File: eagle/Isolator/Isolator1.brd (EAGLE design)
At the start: 100 x 80 mm, 15 parts, among them J1 61300411121, J2 61300411121, J4 PJ-102A, Q1 BC557C, Q2 BC557C

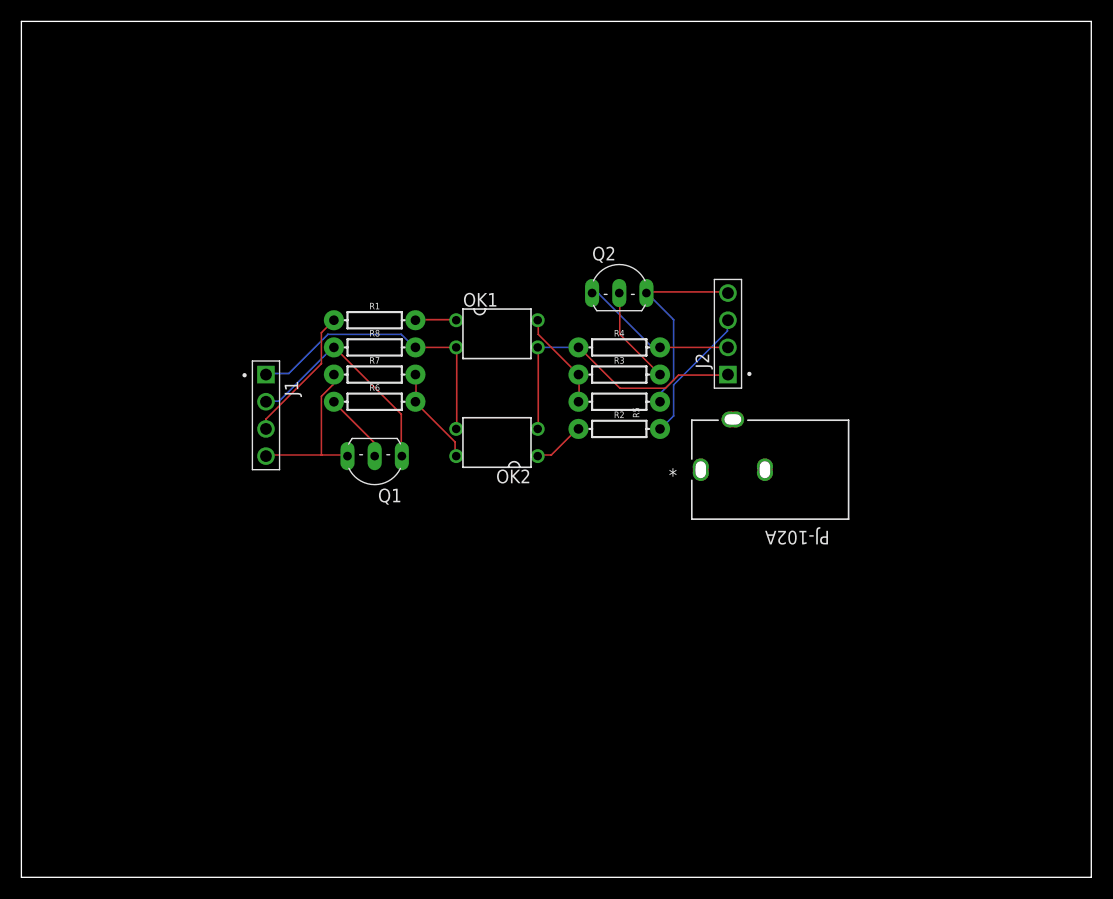
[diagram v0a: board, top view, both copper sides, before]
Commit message: Working - check power jack
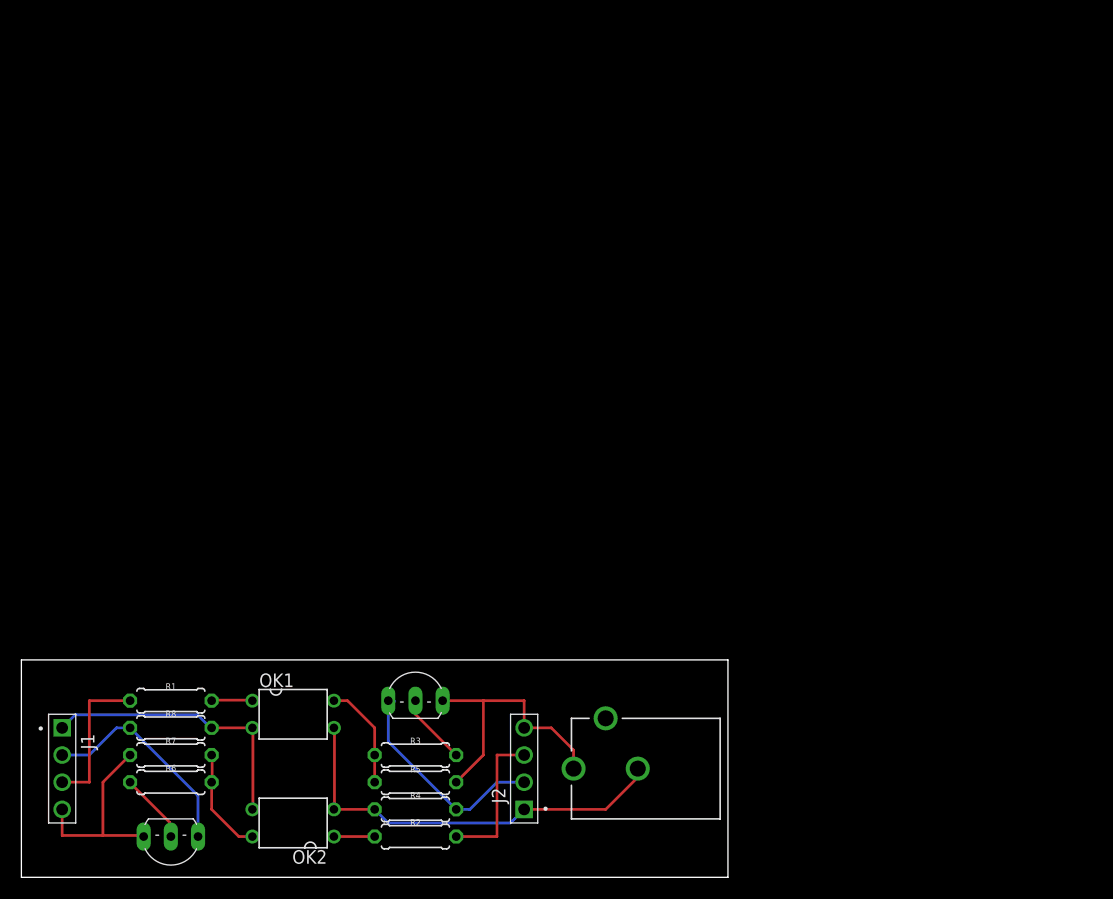
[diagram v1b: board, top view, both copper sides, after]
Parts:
- removed J4: PJ-102A, jack:PJ-102A_CUD
- added U$1: CUI_PJ-102A, con-dc-jack:CUI_DCJACK_PCB
- OK1, OK2: value SFH618A-2 -> SFH617A-2
- Q1, Q2: value BC557C -> 2N3906
- R1, R2: value (none) -> 200; device SparkFun-Resistors:AXIAL-0.3 -> resistor:0207/7
- R3, R6: value (none) -> 1500; device SparkFun-Resistors:AXIAL-0.3 -> resistor:0207/7
- R4, R8: value (none) -> 1000; device SparkFun-Resistors:AXIAL-0.3 -> resistor:0207/7
- R5, R7: value (none) -> 75; device SparkFun-Resistors:AXIAL-0.3 -> resistor:0207/7
- moved R4 47.2 mm to (36.8, 6.35)
- moved J2 44.9 mm to (47.0, 10.2)
- moved Q2 42.6 mm to (36.8, 17.8)
- moved R2 42.6 mm to (36.8, 3.81)
- moved OK1 40.3 mm to (25.4, 15.2)
- moved OK2 40.3 mm to (25.4, 5.08)
- moved Q1 40.3 mm to (14.0, 2.54)
- moved R1 40.3 mm to (14.0, 16.5)
- moved R3 40.3 mm to (36.8, 11.4)
- moved R5 40.3 mm to (36.8, 8.89)
- moved R6 40.3 mm to (14.0, 8.89)
- moved R7 40.3 mm to (14.0, 11.4)
- moved R8 40.3 mm to (14.0, 14.0)
- moved J1 38.1 mm to (3.81, 10.2)
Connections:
- new net CASE: U$1.CASE
- net GND1: now also R8.2; no longer R8.P$2
- net GND2: now also R4.1, U$1.-; no longer J4.2, J4.3, R4.P$1
- net N$1: now also R2.1; no longer R2.P$1
- net N$2: now also R3.1, R5.2; no longer R3.P$1, R5.P$2
- net N$3: now also R3.2; no longer R3.P$2
- net N$4: now also R1.2; no longer R1.P$2
- net N$6: now also R6.2, R7.2; no longer R6.P$2, R7.P$2
- net N$7: now also R6.1; no longer R6.P$1
- net RX1: now also R8.1; no longer R8.P$1
- net RX2: now also R4.2; no longer R4.P$2
- net TX1: now also R1.1; no longer R1.P$1
- net TX2: now also R2.2; no longer R2.P$2
- net VCC1: now also R7.1; no longer R7.P$1
- net VCC2: now also R5.1, U$1.+; no longer J4.1, R5.P$1
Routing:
- net GND2: track 28.8 -> 39.2 mm
- net VCC2: track 19.5 -> 26.2 mm, vias 2 -> 0
- net RX2: track 14.8 -> 20.8 mm
- net VCC1: track 15.8 -> 18.8 mm
- net N$3: track 9.20 -> 6.73 mm
- net N$2: track 9.23 -> 10.6 mm
- net TX2: track 12.8 -> 14.0 mm
- net TX1: track 12.8 -> 14.0 mm
- net GND1: track 27.6 -> 26.6 mm
- net N$6: track 9.23 -> 10.2 mm
- net RX1: track 21.3 -> 20.5 mm
- net N$1: track 4.88 -> 4.29 mm
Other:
- board size 100 x 80 mm -> 66 x 20.3 mm
- board text added: "Gnd1"
- board text added: "Gnd2"
- board text added: "Rx1"
- board text added: "Rx2"
- board text added: "Serial Opto-isolator v1.0 Copyright (c) 2022 Whitmer Consulting LLC"
- board text added: "Tx1"
- board text added: "Tx2"
- board text added: "Vcc1"
- board text added: "Vcc2"
- board text added: "Vcc2 5V"
